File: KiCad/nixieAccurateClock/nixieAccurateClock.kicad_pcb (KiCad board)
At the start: 2 copper layers, 221 x 109.2 mm, 17 parts, among them J1 Conn_01x02_Pin, J2 Conn_01x02_Pin, J3 Conn_01x02_Pin, J4 Conn_Coaxial, Q1 PZTA42, SW1 SW_DIP_x02, U2 PX1125T

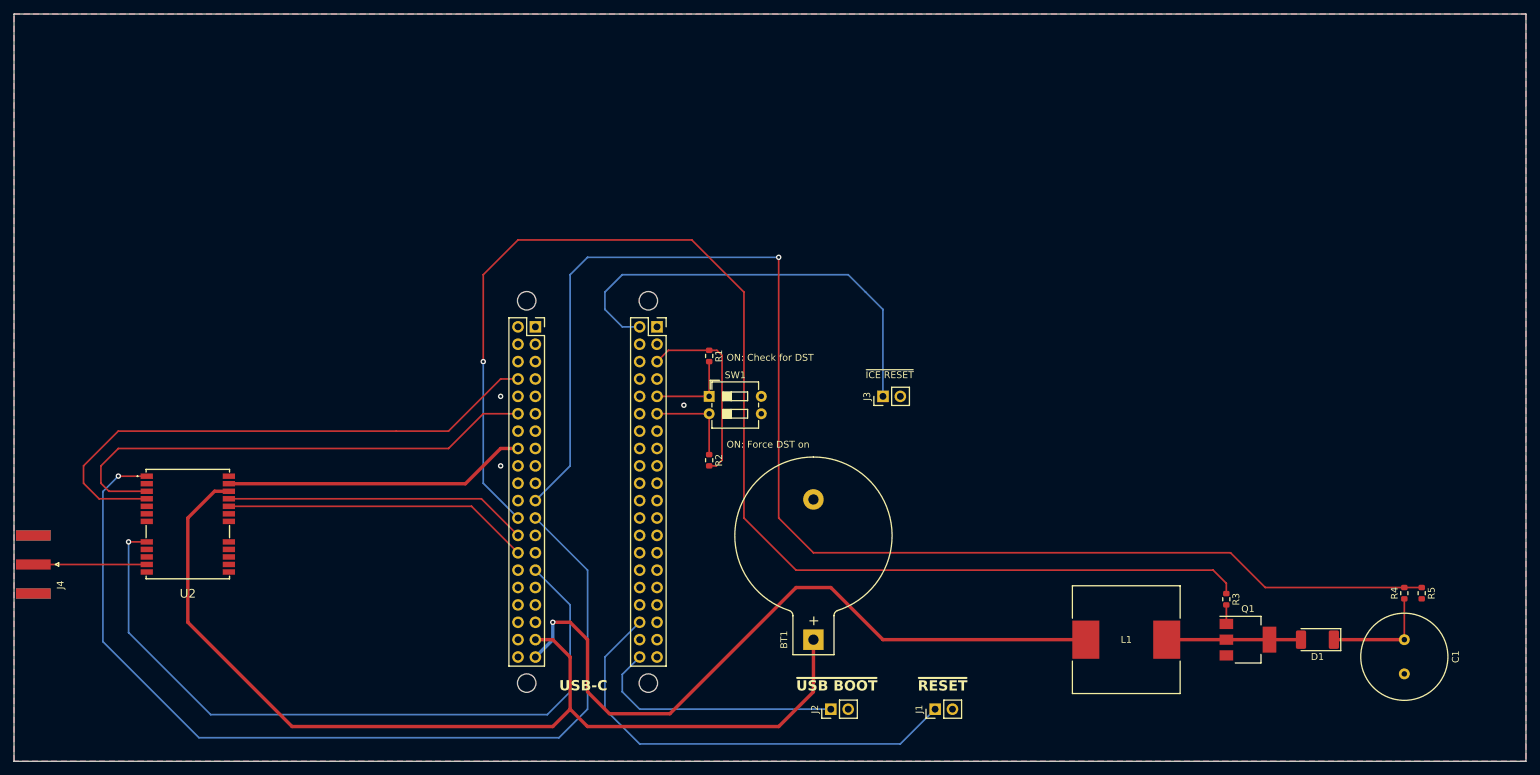
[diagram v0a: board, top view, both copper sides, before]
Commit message: WIP nixies
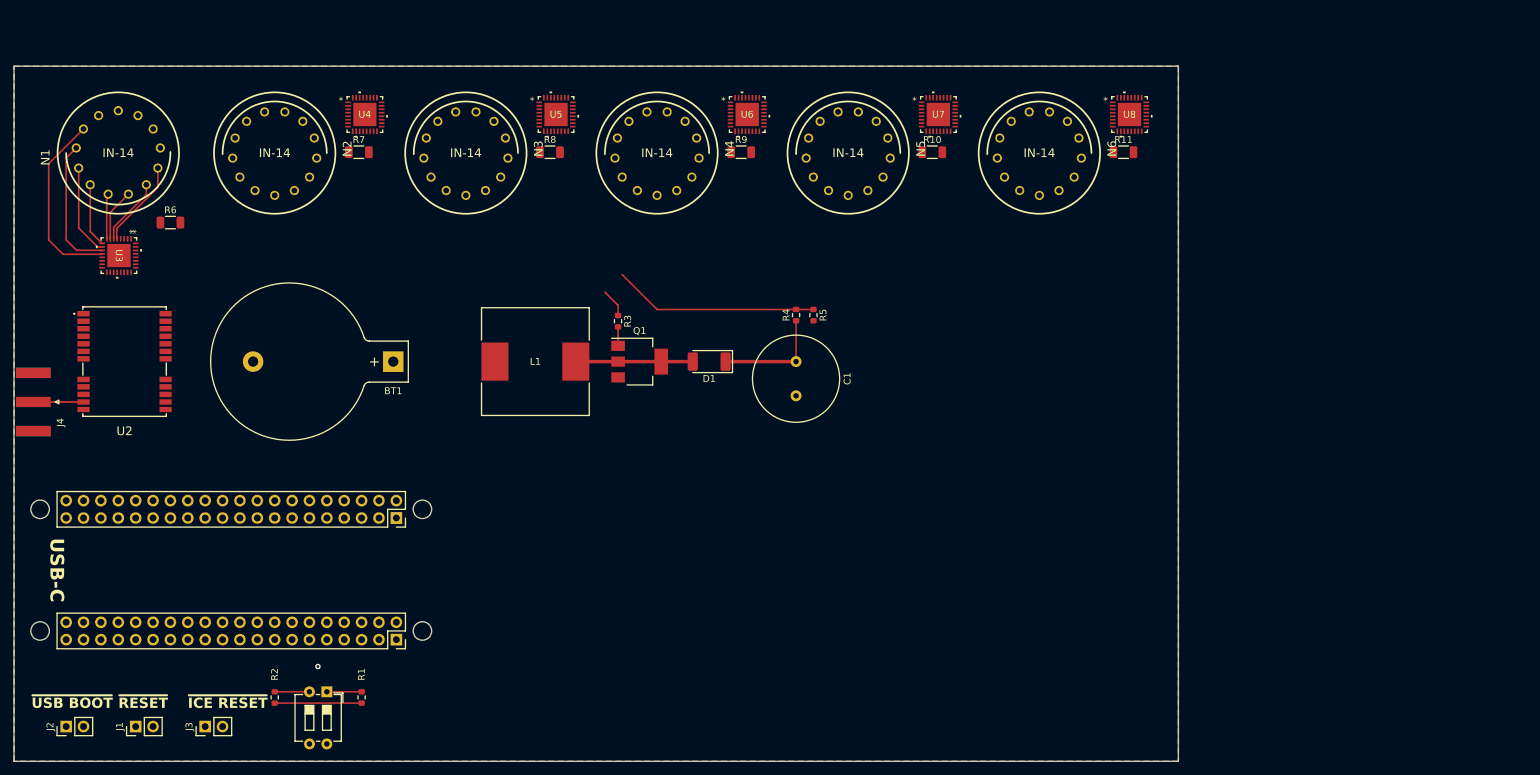
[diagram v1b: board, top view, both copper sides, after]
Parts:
- added N1: IN-14, 00_lib:nixies-us-IN-14, F.Cu at (40.6, 38.1)
- added N2: IN-14, 00_lib:nixies-us-IN-14, F.Cu at (63.5, 38.1)
- added N3: IN-14, 00_lib:nixies-us-IN-14, F.Cu at (91.4, 38.1)
- added N4: IN-14, 00_lib:nixies-us-IN-14, F.Cu at (119.4, 38.1)
- added N5: IN-14, 00_lib:nixies-us-IN-14, F.Cu at (147.3, 38.1)
- added N6: IN-14, 00_lib:nixies-us-IN-14, F.Cu at (175.3, 38.1)
- added R10: 33k, Resistor_SMD:R_1206_3216Metric, F.Cu at (159.6, 38.0)
- added R11: 33k, Resistor_SMD:R_1206_3216Metric, F.Cu at (187.6, 38.0)
- added R6: 33k, Resistor_SMD:R_1206_3216Metric, F.Cu at (48.3, 48.3)
- added R7: 33k, Resistor_SMD:R_1206_3216Metric, F.Cu at (75.8, 38.0)
- added R8: 33k, Resistor_SMD:R_1206_3216Metric, F.Cu at (103.7, 38.0)
- added R9: 33k, Resistor_SMD:R_1206_3216Metric, F.Cu at (131.7, 38.0)
- added U3: HV509K6-G, 00_lib:QFN32_5X5MC_MCH, F.Cu at (40.7, 53.1)
- added U4: HV509K6-G, 00_lib:QFN32_5X5MC_MCH, F.Cu at (76.7, 32.5)
- added U5: HV509K6-G, 00_lib:QFN32_5X5MC_MCH, F.Cu at (104.6, 32.5)
- added U6: HV509K6-G, 00_lib:QFN32_5X5MC_MCH, F.Cu at (132.6, 32.5)
- added U7: HV509K6-G, 00_lib:QFN32_5X5MC_MCH, F.Cu at (160.5, 32.5)
- added U8: HV509K6-G, 00_lib:QFN32_5X5MC_MCH, F.Cu at (188.4, 32.5)
- moved J1 116.9 mm to (43.2, 121.9)
- moved J2 111.8 mm to (33.0, 121.9)
- moved J3 110.2 mm to (53.3, 121.9)
- moved C1 97.7 mm to (139.7, 68.6)
- moved D1 97.7 mm to (127.0, 68.6)
- moved Q1 97.7 mm to (116.8, 68.6)
- moved R4 97.7 mm to (139.7, 61.8)
- moved R3 97.7 mm to (113.7, 62.7)
- moved R5 97.7 mm to (142.2, 61.8)
- moved L1 95.4 mm to (101.6, 68.6)
- moved BT1 73.6 mm to (80.8, 68.6), turned to 180 degrees
- moved R2 72.3 mm to (63.5, 117.7)
- moved R1 71.2 mm to (76.2, 117.7), turned to 90 degrees
- moved SW1 70.6 mm to (71.1, 116.8), turned to -90 degrees
- moved U1 52.4 mm to (58.4, 99.1), turned to -90 degrees
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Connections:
- net Net-(D1-K) renamed VPP
- U1 pad 13: unconnected-(U1-ICE_36-Pad13) -> PPS_TRIMMED
- U1 pad 14: unconnected-(U1-ICE_38-Pad14) -> HV_CLOCK
- U1 pad 15: unconnected-(U1-ICE_42-Pad15) -> HV_POLARITY
- U1 pad 16: unconnected-(U1-ICE_43-Pad16) -> HV_DATA
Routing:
- net HV_GATE: track 190.0 -> 4.26 mm, vias 1 -> 0
- net HV_SENSE: track 202.9 -> 30.0 mm, vias 1 -> 0
- net +3V3_STDBY: track 146.2 -> 0.00 mm
- net GPS_BOOT_SEL: track 138.8 -> 0.00 mm, vias 1 -> 0
- net GPS_RSTN: track 106.7 -> 0.00 mm, vias 1 -> 0
- net +5V: track 104.8 -> 0.00 mm, vias 1 -> 0
- net GPS_1PPS2: track 81.5 -> 0.00 mm
- net GPS_1PPS: track 73.8 -> 0.00 mm
- net /~{RESET}: track 67.3 -> 0.00 mm
- net /~{ICE_RST}: track 65.2 -> 0.00 mm
- net +3.3V: track 72.4 -> 12.7 mm
- net GPS_TXD: track 45.1 -> 0.00 mm
- net GPS_RXD: track 44.5 -> 0.00 mm
- net /~{USB_BOOT}: track 37.7 -> 0.00 mm
- net /Nixies/Nixie1/N_1: track 0.00 -> 27.0 mm
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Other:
- board size 221 x 109.2 mm -> 170.2 x 101.6 mm
- board text removed: "ON: Check for DST"
- board text removed: "ON: Force DST on"
- board text removed: "USB-C"
